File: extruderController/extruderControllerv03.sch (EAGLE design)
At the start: 76 parts, among them IC1 LM1117MPX-5.0, IC2 MAX3467CPA, IC3 ATMEGA2561-16AU, IC4 ULN2003AD, J8 615016137621, Q2 PH7030L, Q3 PH7030L, Q4 PH7030L, Q5 PH7030L, Q6 PH7030L, X1 22-23-2081, X2 22-23-2081, X3 22-23-2101, X4 22-23-2051, X8 22-23-2031, X9 22-23-2031

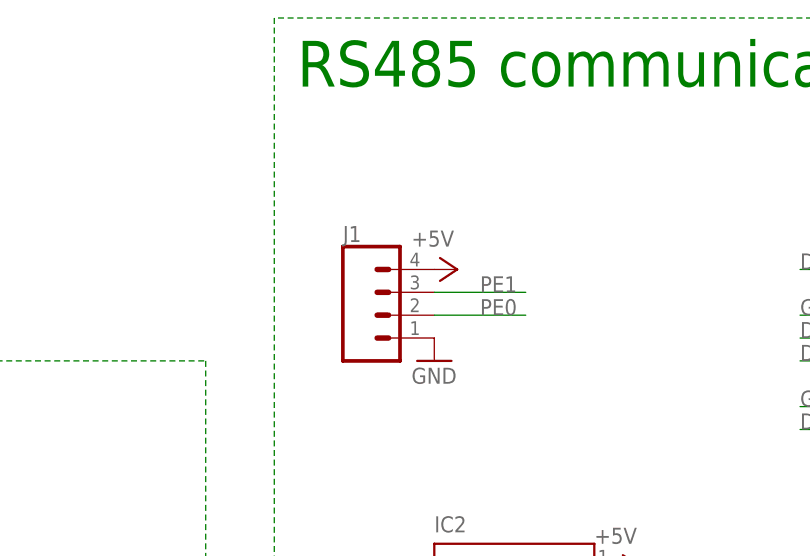
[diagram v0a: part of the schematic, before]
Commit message: f
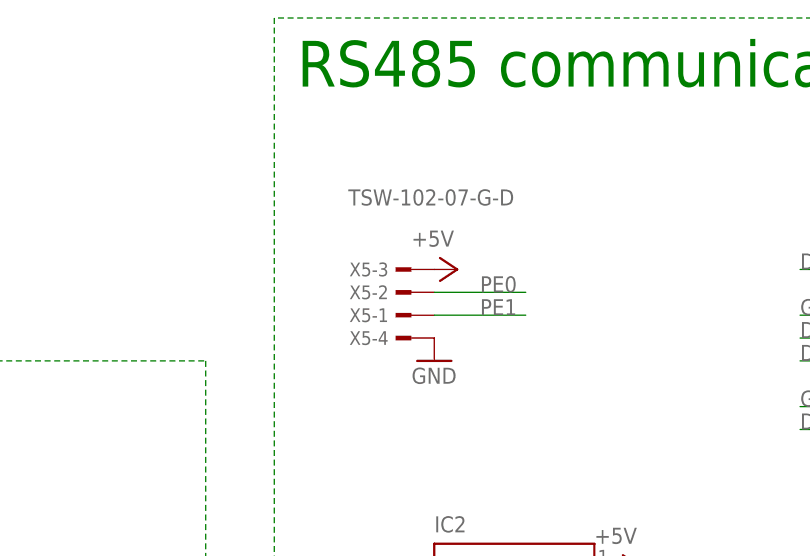
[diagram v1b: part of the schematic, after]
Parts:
- removed J1: (no value), SparkFun-Connectors:CONN_04
- added X5: TSW-102-07-G-D, con-samtec:TSW-102-07-G-D
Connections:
- net +5V: now also X5-3.1; no longer J1.4
- net GND: now also X5-4.1; no longer J1.1
- net PE0: now also X5-2.1; no longer J1.2
- net PE1: now also X5-1.1; no longer J1.3
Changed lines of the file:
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@@
 <part name="J8" library="SamacSys_Parts" deviceset="615016137621" device=""/>
 <part name="R12" library="rcl" library_urn="urn:adsk.eagle:library:334" deviceset="R-EU_" device="R1210" package3d_urn="urn:adsk.eagle:package:23554/2" value="120"/>
-<part name="J1" library="SparkFun-Connectors" library_urn="urn:adsk.eagle:library:513" deviceset="CONN_04" device="" package3d_urn="urn:adsk.eagle:package:38085/1"/>
 <part name="GND24" library="supply1" library_urn="urn:adsk.eagle:library:371" deviceset="GND" device=""/>
 <part name="P+34" library="supply1" library_urn="urn:adsk.eagle:library:371" deviceset="+5V" device=""/>
@@
 <part name="R20" library="rcl" library_urn="urn:adsk.eagle:library:334" deviceset="R-EU_" device="R0805" package3d_urn="urn:adsk.eagle:package:23553/2" value="27"/>
 <part name="X4" library="con-molex" library_urn="urn:adsk.eagle:library:165" deviceset="22-23-2051" device=""/>
+<part name="X5" library="con-samtec" library_urn="urn:adsk.eagle:library:184" deviceset="TSW-102-*-G" device="-D" technology="07"/>
 </parts>
 <sheets>
@@
 <attribute name="VALUE" x="123.19" y="179.578" size="1.778" layer="96"/>
 </instance>
-<instance part="J1" gate="G$1" x="76.2" y="231.14" smashed="yes">
-<attribute name="VALUE" x="71.12" y="223.774" size="1.778" layer="96" font="vector"/>
-<attribute name="NAME" x="71.12" y="239.268" size="1.778" layer="95" font="vector"/>
-</instance>
 <instance part="GND24" gate="1" x="81.28" y="226.06" smashed="yes">
 <attribute name="VALUE" x="78.74" y="223.52" size="1.778" layer="96"/>
@@
 <instance part="X4" gate="-5" x="-139.7" y="165.1" smashed="yes" rot="R180">
 <attribute name="NAME" x="-142.24" y="165.862" size="1.524" layer="95" rot="R180"/>
+</instance>
+<instance part="X5" gate="-1" x="78.74" y="231.14" smashed="yes" rot="R180">
+<attribute name="VALUE" x="90.17" y="245.11" size="1.778" layer="96" rot="R180"/>
+<attribute name="NAME" x="76.2" y="231.902" size="1.524" layer="95" rot="R180"/>
+</instance>
+<instance part="X5" gate="-2" x="78.74" y="233.68" smashed="yes" rot="R180">
+<attribute name="NAME" x="76.2" y="234.442" size="1.524" layer="95" rot="R180"/>
+</instance>
+<instance part="X5" gate="-3" x="78.74" y="236.22" smashed="yes" rot="R180">
+<attribute name="NAME" x="76.2" y="236.982" size="1.524" layer="95" rot="R180"/>
+</instance>
+<instance part="X5" gate="-4" x="78.74" y="228.6" smashed="yes" rot="R180">
+<attribute name="NAME" x="76.2" y="229.362" size="1.524" layer="95" rot="R180"/>
 </instance>
 </instances>
@@
 </segment>
 <segment>
-<pinref part="J1" gate="G$1" pin="1"/>
-<pinref part="GND24" gate="1" pin="GND"/>
-</segment>
-<segment>
 <pinref part="GND13" gate="1" pin="GND"/>
 <pinref part="C4" gate="G$1" pin="2"/>
@@
 <pinref part="GND20" gate="1" pin="GND"/>
 <pinref part="X4" gate="-5" pin="S"/>
+</segment>
+<segment>
+<pinref part="GND24" gate="1" pin="GND"/>
+<pinref part="X5" gate="-4" pin="1"/>
 </segment>
 </net>
@@
 </segment>
 <segment>
-<pinref part="J1" gate="G$1" pin="4"/>
 <pinref part="P+34" gate="1" pin="+5V"/>
+<pinref part="X5" gate="-3" pin="1"/>
 </segment>
 </net>
@@
 </segment>
 <segment>
-<pinref part="J1" gate="G$1" pin="3"/>
-<wire x1="81.28" y1="233.68" x2="91.44" y2="233.68" width="0.1524" layer="91"/>
-<label x="86.36" y="233.68" size="1.778" layer="95"/>
+<wire x1="81.28" y1="231.14" x2="91.44" y2="231.14" width="0.1524" layer="91"/>
+<label x="86.36" y="231.14" size="1.778" layer="95"/>
+<pinref part="X5" gate="-1" pin="1"/>
 </segment>
 </net>
@@
 </segment>
 <segment>
-<pinref part="J1" gate="G$1" pin="2"/>
-<wire x1="81.28" y1="231.14" x2="91.44" y2="231.14" width="0.1524" layer="91"/>
-<label x="86.36" y="231.14" size="1.778" layer="95"/>
-</segment>
-</net>
+<wire x1="81.28" y1="233.68" x2="91.44" y2="233.68" width="0.1524" layer="91"/>
+<label x="86.36" y="233.68" size="1.778" layer="95"/>
+<pinref part="X5" gate="-2" pin="1"/>
+</segment>
+</net>

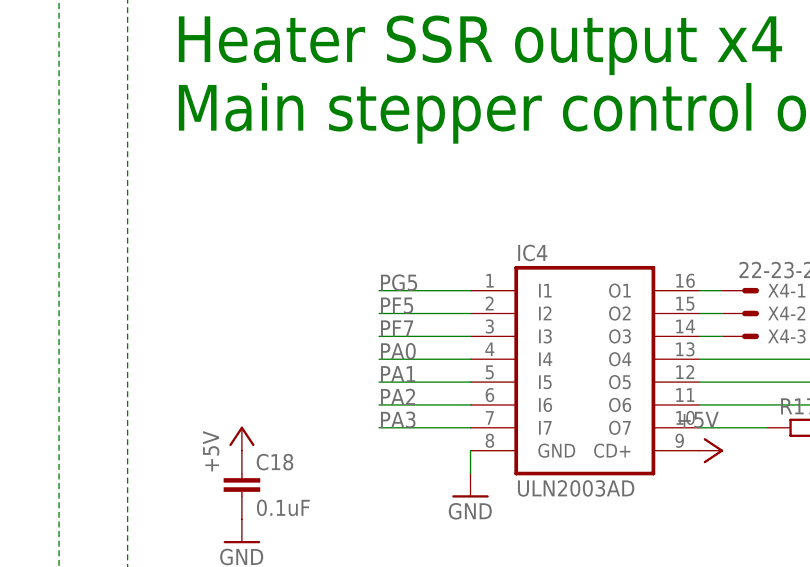
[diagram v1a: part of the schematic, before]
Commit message: e
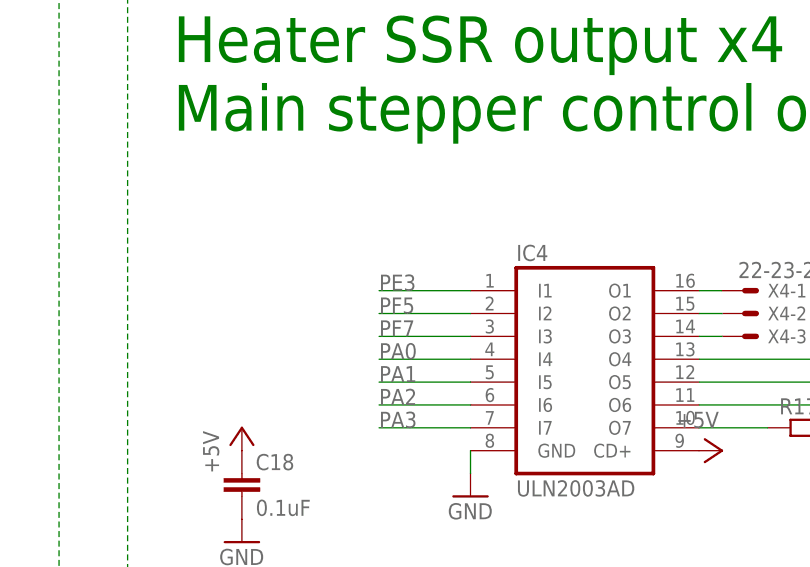
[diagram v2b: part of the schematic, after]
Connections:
- net PE3: now also IC4.I1
- net PG5: no longer IC4.I1
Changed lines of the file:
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@@
 <label x="12.7" y="-10.16" size="1.778" layer="95"/>
-</segment>
-<segment>
-<pinref part="IC4" gate="A" pin="I1"/>
-<wire x1="-210.82" y1="193.04" x2="-220.98" y2="193.04" width="0.1524" layer="91"/>
-<label x="-220.98" y="193.04" size="1.778" layer="95"/>
 </segment>
 </net>
@@
 <label x="30.48" y="25.4" size="1.778" layer="95"/>
 </segment>
+<segment>
+<pinref part="IC4" gate="A" pin="I1"/>
+<wire x1="-210.82" y1="193.04" x2="-220.98" y2="193.04" width="0.1524" layer="91"/>
+<label x="-220.98" y="193.04" size="1.778" layer="95"/>
+</segment>
 </net>
